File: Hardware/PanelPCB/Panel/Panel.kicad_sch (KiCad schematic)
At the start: 15 parts, among them J1 RJ45, J2 Conn_01x03_Socket, U1 AP2204R-5.0, U2 SN74LV1T34DBV

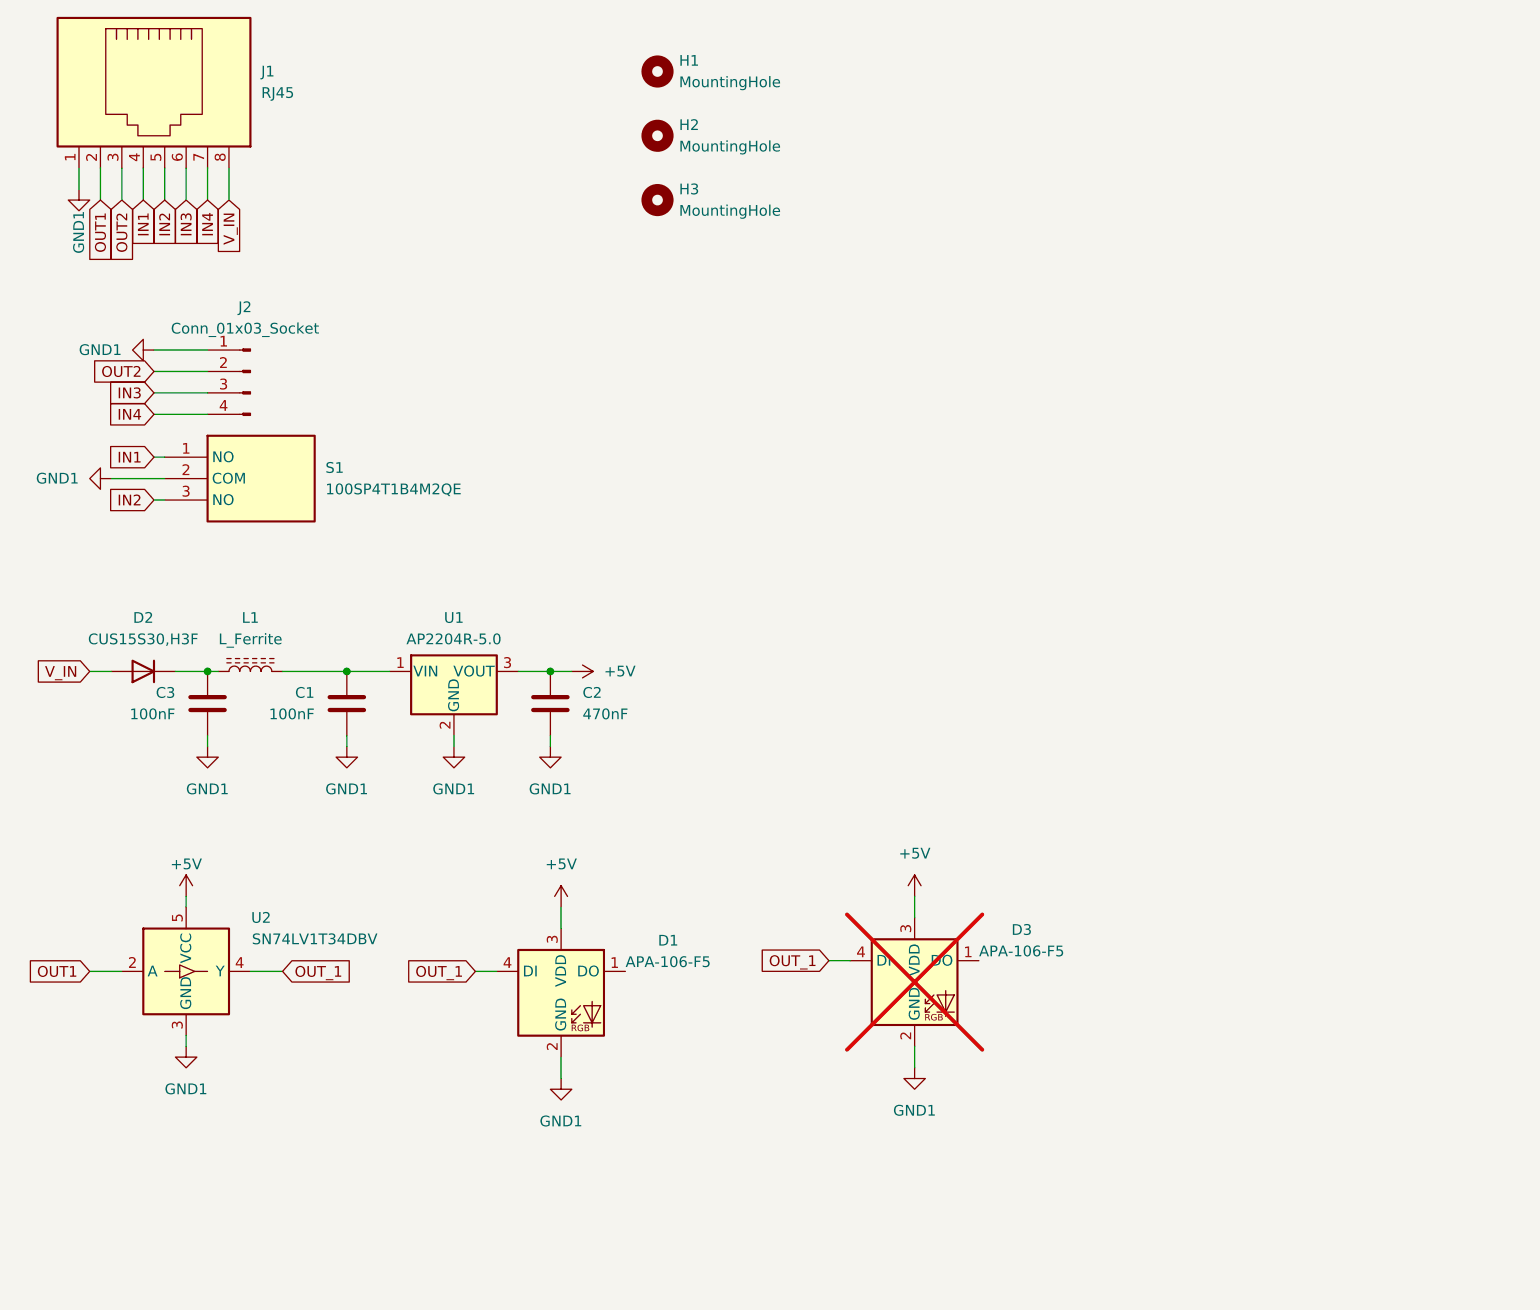
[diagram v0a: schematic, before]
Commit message: update BOM
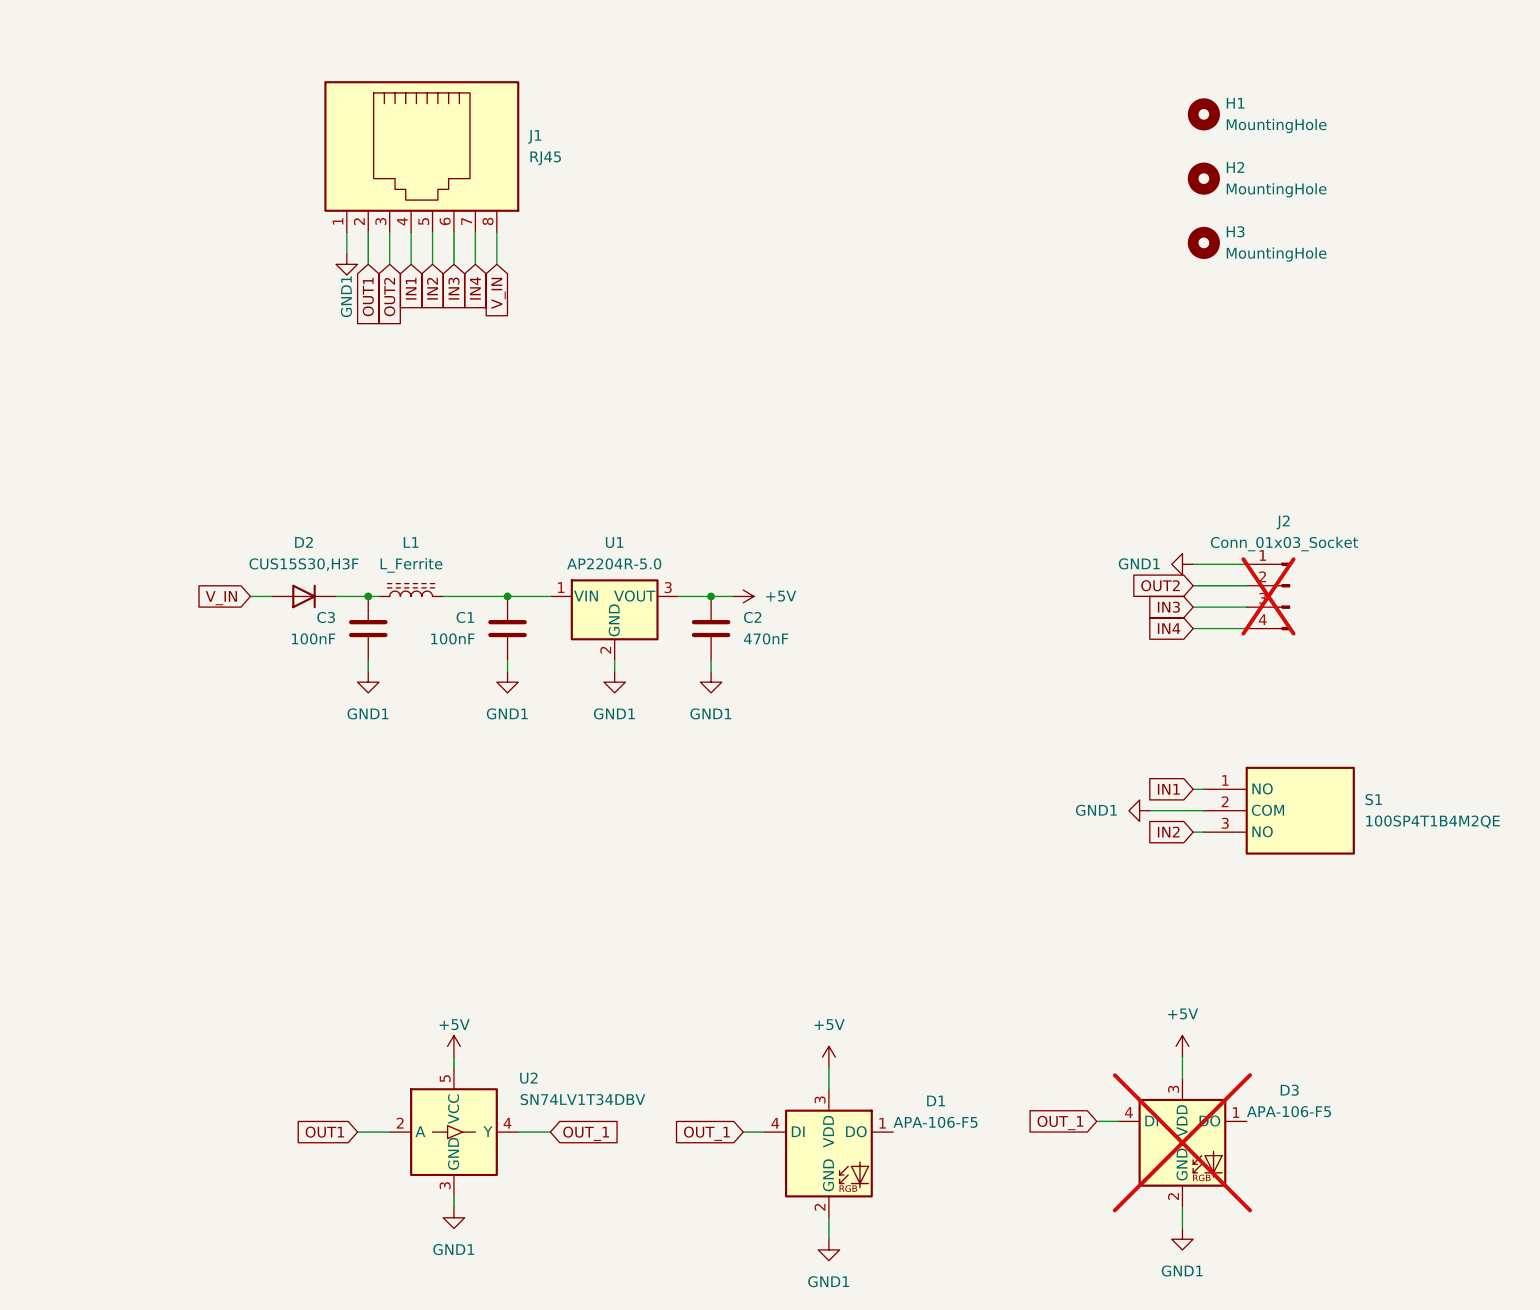
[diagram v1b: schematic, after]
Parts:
- C1, C3: Manufacturer_Name (none) -> Samsung Electro-Mechanics; Manufacturer_Part_Number (none) -> CL10B104KB8NNNC; Mouser Part Number (none) -> 187-CL10B104KB8NNNC
- C2: Manufacturer_Name (none) -> Samsung Electro-Mechanics; Manufacturer_Part_Number (none) -> CL10B474KA8NFNC; Mouser Part Number (none) -> 187-CL10B474KA8NFNC; Mouser Price/Stock (none) -> 0,038 €
- D1: Manufacturer_Name (none) -> SparkFun; Manufacturer_Part_Number (none) -> APA-106-F5
- D2: Manufacturer_Name (none) -> Toshiba; Manufacturer_Part_Number (none) -> CUS15S30,H3F; Mouser Part Number (none) -> 757-CUS15S30H3F; Mouser Price/Stock (none) -> 0,209 €
- D3: Manufacturer_Name (none) -> SparkFun; Manufacturer_Part_Number (none) -> APA-106-F5; now left out of the parts list
- H1, H2, H3: now left out of the parts list
- J1: Manufacturer_Name (none) -> GCT; Manufacturer_Part_Number (none) -> MJ3415-88-2; Mouser Part Number (none) -> 640-MJ3415-88-2; Mouser Price/Stock (none) -> 0,599 €
- J2: now not fitted; now left out of the parts list
- L1: Manufacturer_Name (none) -> Vishay / Dale; Manufacturer_Part_Number (none) -> ILBB0805ER151V; Mouser Part Number (none) -> 70-ILBB0805ER151V; Mouser Price/Stock (none) -> 0,095 €
- S1: Mouser Price/Stock https://www.mouser.com/Search/Refine.aspx?Keyword=612-100SP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 -> (none)
- U1: Mouser Part Number (none) -> 621-AP2204R-5.0TRG1; Price 1€ -> (none)
- U2: Price 0,4€ -> (none)
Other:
- moved on the sheet: C1, C2, C3, D1, D2, D3, H1, H2, H3, J1, L1, S1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
